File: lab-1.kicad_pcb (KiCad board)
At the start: 2 copper layers, 39.5 x 59.5 mm, 31 parts, among them J1 Conn_01x04_Pin, J2 USB_C_Receptacle, SW1 NRST, SW2 BOOT, U1 LM66100DCK, U2 LM66100DCK, U3 STM32F405RGTx, U4 MCP1700x-120xxMB, Y1 8 MHz

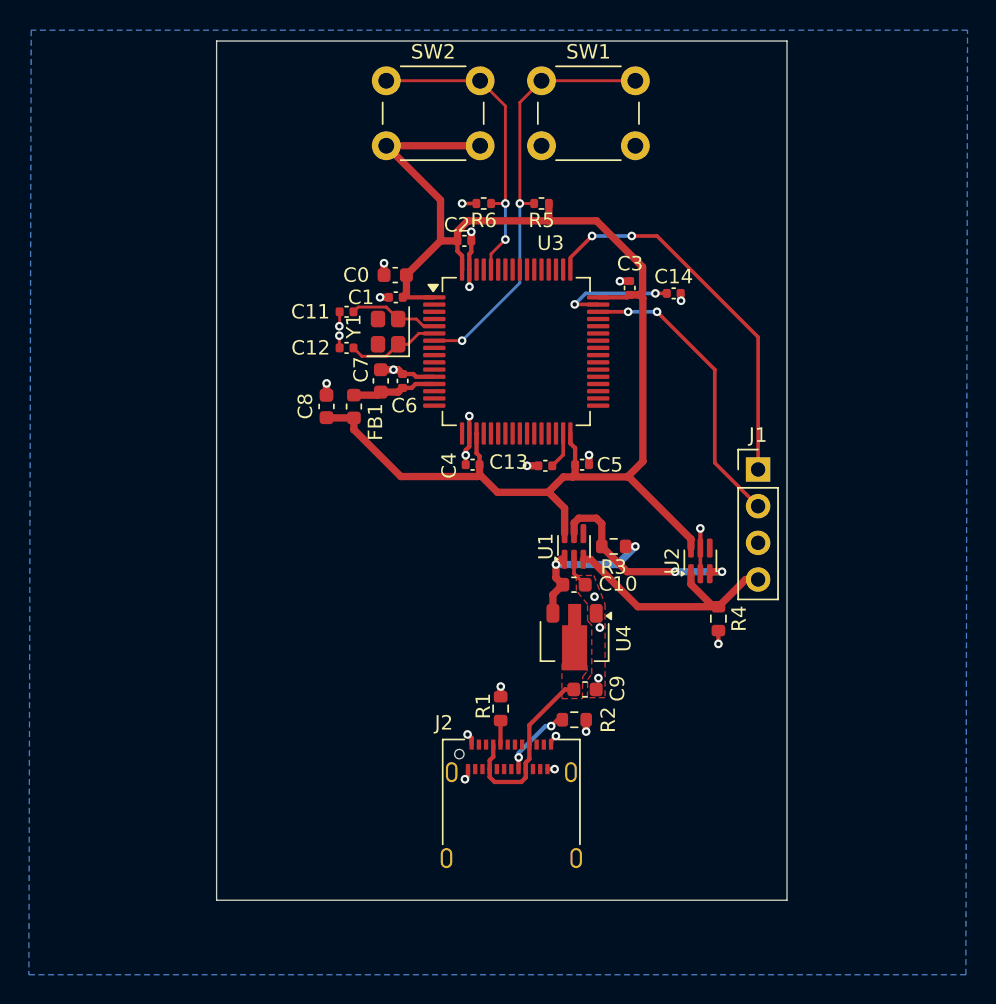
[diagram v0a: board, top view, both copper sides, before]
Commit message: minor adjustments
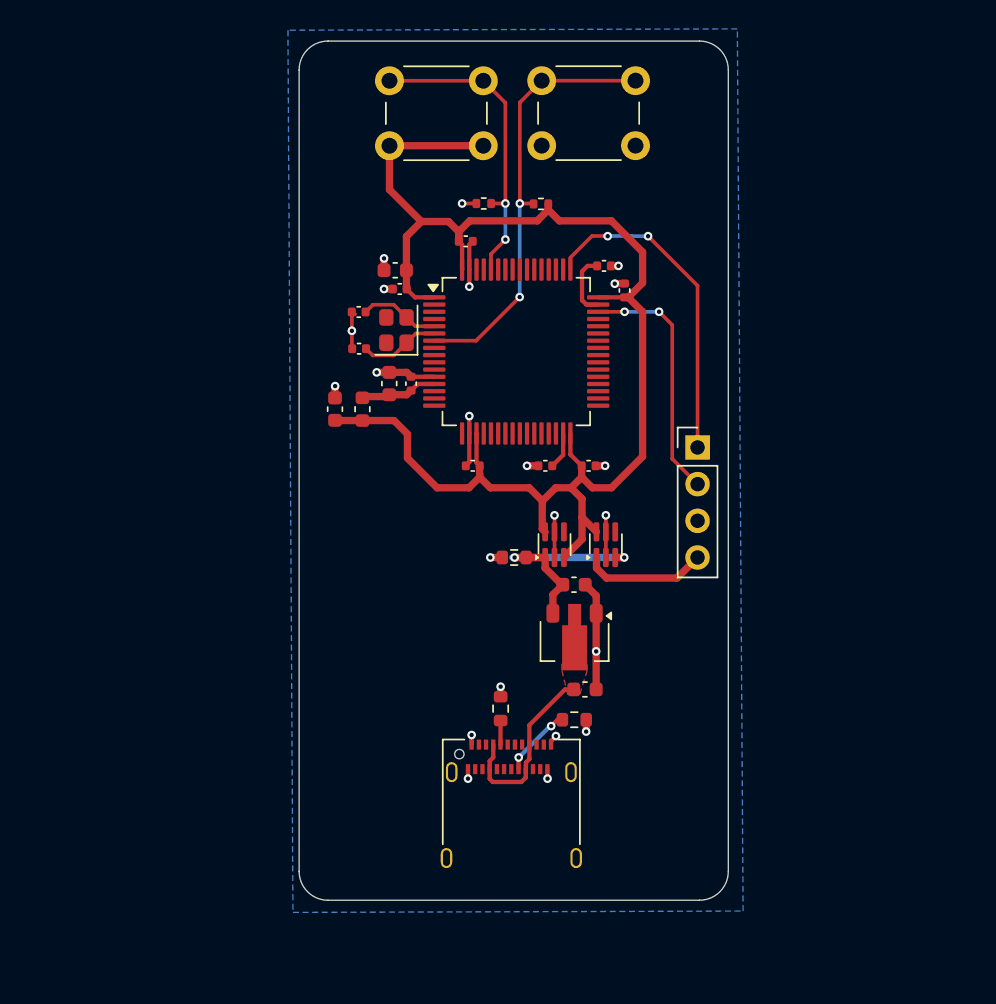
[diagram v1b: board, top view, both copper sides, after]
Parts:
- removed R4: 100k, Resistor_SMD:R_0603_1608Metric
- moved R3 6.94 mm to (157.6, 112.0), turned to 0 degrees
- moved U2 6.64 mm to (164.0, 111.1)
- moved C14 5.19 mm to (163.8, 91.8)
- moved J1 4.46 mm to (170.3, 104.4)
- moved U1 1.35 mm to (160.4, 111.1)
- moved C12 0.87 mm to (146.9, 97.6)
- moved C11 0.84 mm to (146.8, 95.0)
- moved C1 0.64 mm to (149.7, 93.4)
- moved C6 0.62 mm to (150.5, 100.0)
- moved FB1 0.62 mm to (147.1, 101.7)
- moved C7 0.62 mm to (149.0, 100.0)
- moved C8 0.62 mm to (145.2, 101.7)
- moved Y1 0.59 mm to (149.5, 96.3)
- moved C5 0.46 mm to (162.8, 105.7)
- moved C3 0.40 mm to (165.3, 93.5)
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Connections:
- R3 pad 1: +3.3V_LDO -> GND
- R3 pad 2: Net-(U1-ST) -> +3.3V_LDO
- U1 pad 3: +3.3V_STLINK -> +3.3V
- U1 pad 5: Net-(U1-ST) -> GND
- U2 pad 3: Net-(U1-ST) -> +3.3V_LDO
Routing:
- net Net-(U1-ST): track 14.5 -> 0.00 mm, vias 2 -> 0
- net +3.3V_STLINK: track 17.5 -> 8.61 mm
- net GND: track 29.7 -> 38.0 mm, vias 26 -> 22
- net Net-(U3-VCAP_2): track 8.33 -> 4.44 mm, vias 2 -> 0
- net +3.3V_LDO: track 11.2 -> 15.0 mm
- net /SWCLK: track 26.5 -> 22.9 mm
- net /SWDIO: track 20.4 -> 17.3 mm
- net /OSC_OUT: track 6.49 -> 5.55 mm
- net /OSC_IN: track 6.28 -> 5.58 mm
- net /NRST: track 29.7 -> 30.2 mm
- net +3.3V: track 99.9 -> 100.4 mm
- net +3.3VA: track 5.88 -> 5.37 mm
- removed copper zone on F.Cu, net GND
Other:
- board size 39.5 x 59.5 mm -> 29.7 x 59.5 mm
